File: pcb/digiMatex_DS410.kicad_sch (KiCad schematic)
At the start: 49 parts, among them J1 POWER, J2 JTAG, J3 PROG, J4 Buttons, J5 SCALE, Q1 MMBT3904, Q2 MMBT3904, Q3 MMBT3904, SW1 SW_Push, SW2 SW_Push, U1 MAX7219, U2 L7805CDT-TR, U3 ESP32-WROOM-32E, U4 NCP1117DT33G

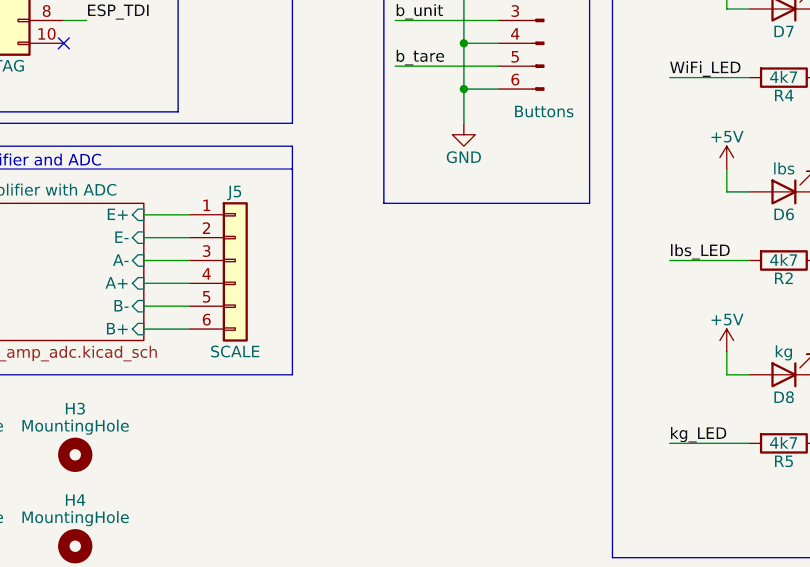
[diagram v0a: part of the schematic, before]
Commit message: add load cell pinout
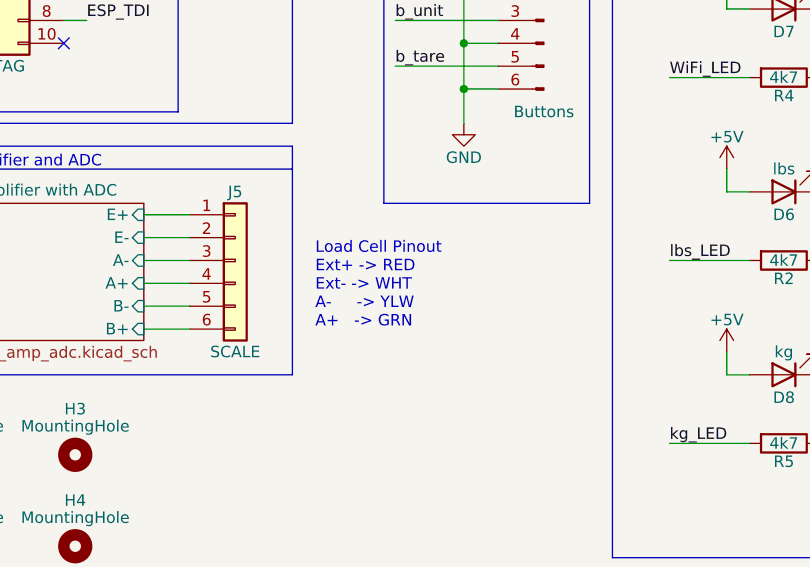
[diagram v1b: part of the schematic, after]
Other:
- note added: "Load Cell Pinout Ext+ -> RED Ext- -> WHT A- -> YLW A+ -> GRN"
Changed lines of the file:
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@@
     (comment 1 "PCB to be maufactured by prototype board house (JLCPCB)")
   )
+  (bus_alias "Buttons" (members "b_display" "b_tare" "b_unit"))
+  (bus_alias "HX711" (members "SCK" "DT"))
+  (bus_alias "MAX7219" (members "CLK" "MOSI" "CS"))
+  (bus_alias "LED" (members "WiFi_LED" "lbs_LED" "kg_LED"))
   (bus_alias "7Seg" (members "A" "B" "C" "D" "E" "F" "G" "DP" "1" "2" "3" "4" "5" "6" "7" "0"))
-  (bus_alias "LED" (members "WiFi_LED" "lbs_LED" "kg_LED"))
-  (bus_alias "MAX7219" (members "CLK" "MOSI" "CS"))
-  (bus_alias "HX711" (members "SCK" "DT"))
-  (bus_alias "Buttons" (members "b_display" "b_tare" "b_unit"))
   (junction (at 110.49 34.29) (diameter 0) (color 0 0 0 0)
   )
@@
     (effects (font (size 1.27 1.27)) (justify left bottom))
   )
+  (text "Load Cell Pinout\nExt+ -> RED\nExt- -> WHT\nA-	 -> YLW\nA+   -> GRN"
+    (at 128.27 139.7 0)
+    (effects (font (size 1.27 1.27)) (justify left bottom))
+  )
